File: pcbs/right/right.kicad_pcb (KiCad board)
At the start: 2 copper layers, 111.6 x 82.4 mm, 53 parts, among them J1 Conn_01x12_Socket

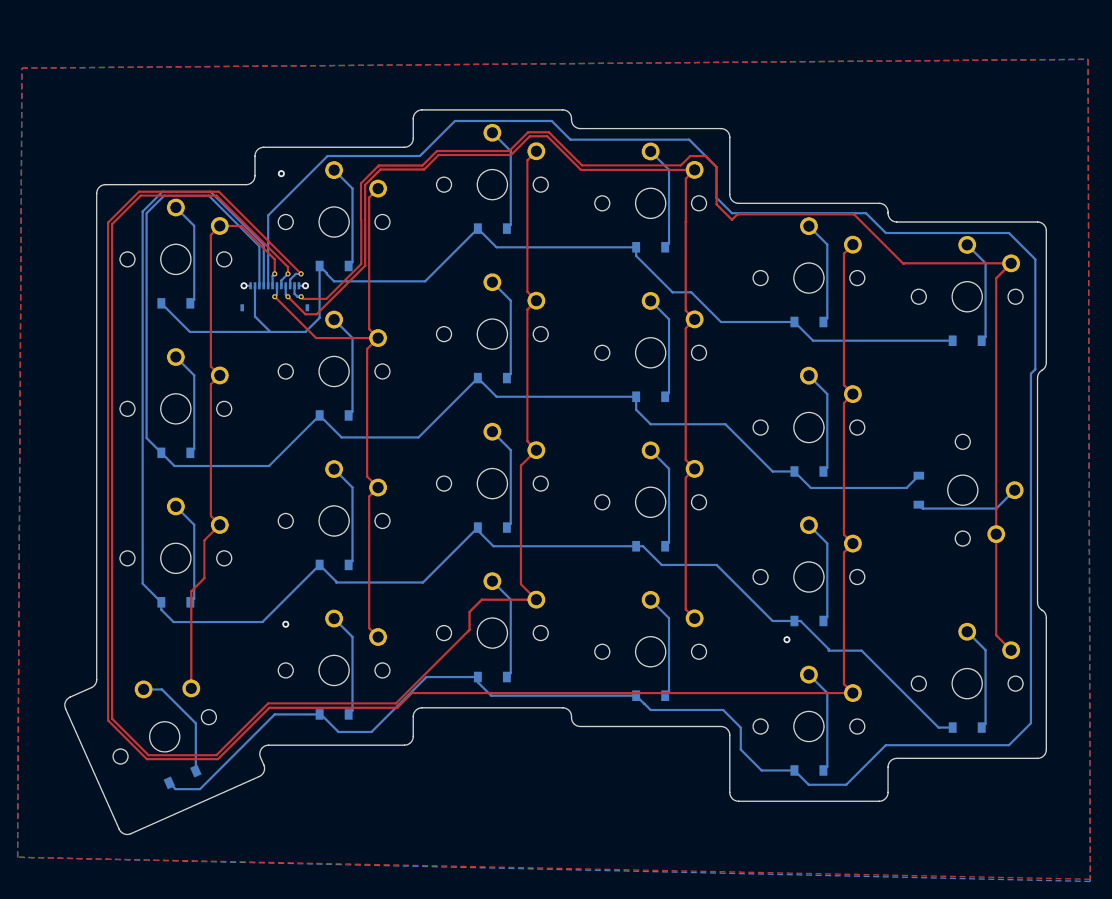
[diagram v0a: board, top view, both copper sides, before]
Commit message: fix offset etc
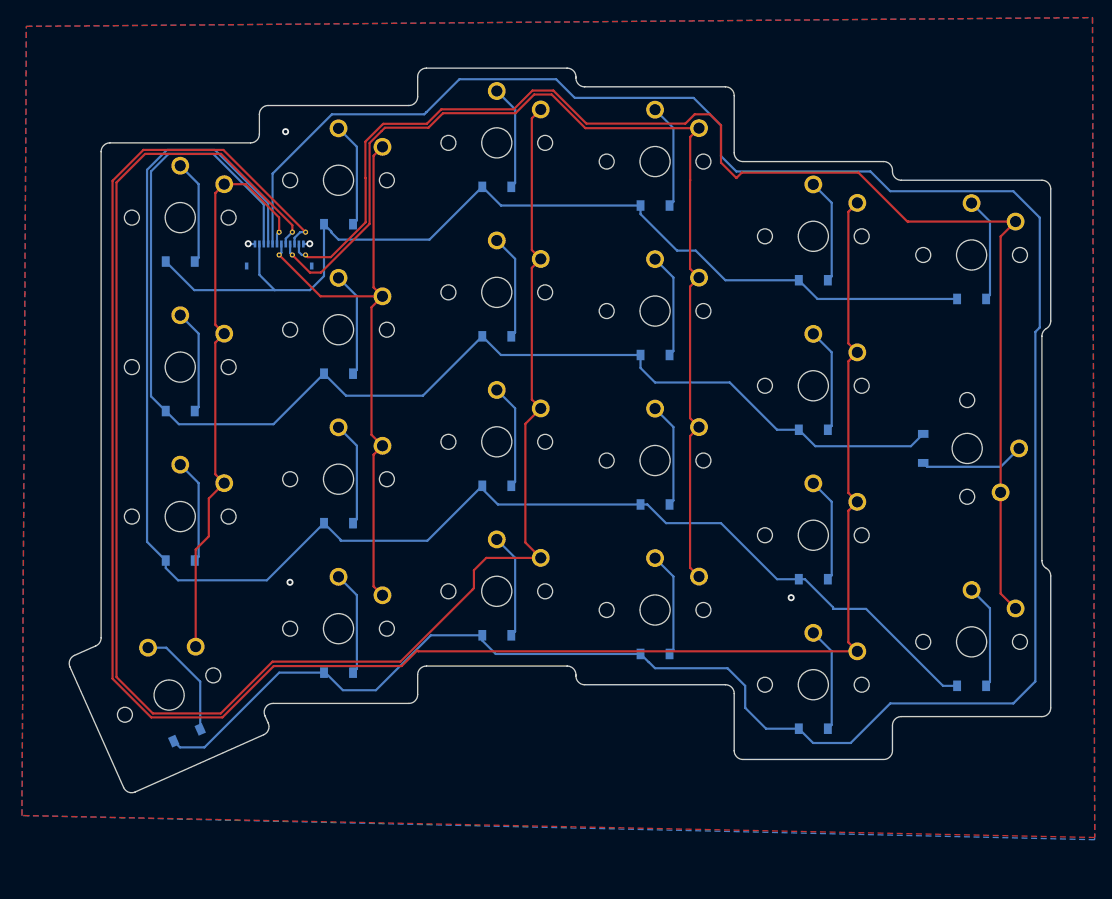
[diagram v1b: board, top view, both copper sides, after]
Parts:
- moved D1 4.78 mm to (316.0, 136.2)
- moved D10 4.78 mm to (280.0, 98.6)
- moved D11 4.78 mm to (280.0, 81.6)
- moved D12 4.78 mm to (262.0, 130.5)
- moved D13 4.78 mm to (262.0, 113.5)
- moved D14 4.78 mm to (262.0, 96.5)
- moved D15 4.78 mm to (262.0, 79.5)
- moved D16 4.78 mm to (244.0, 134.8)
- moved D17 4.78 mm to (244.0, 117.8)
- moved D18 4.78 mm to (244.0, 100.8)
- moved D19 4.78 mm to (244.0, 83.8)
- moved D2 4.78 mm to (310.5, 109.2)
- moved D20 4.78 mm to (226.8, 141.9)
- moved D21 4.78 mm to (226.0, 122.0)
- moved D22 4.78 mm to (226.0, 105.0)
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
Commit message: old changes
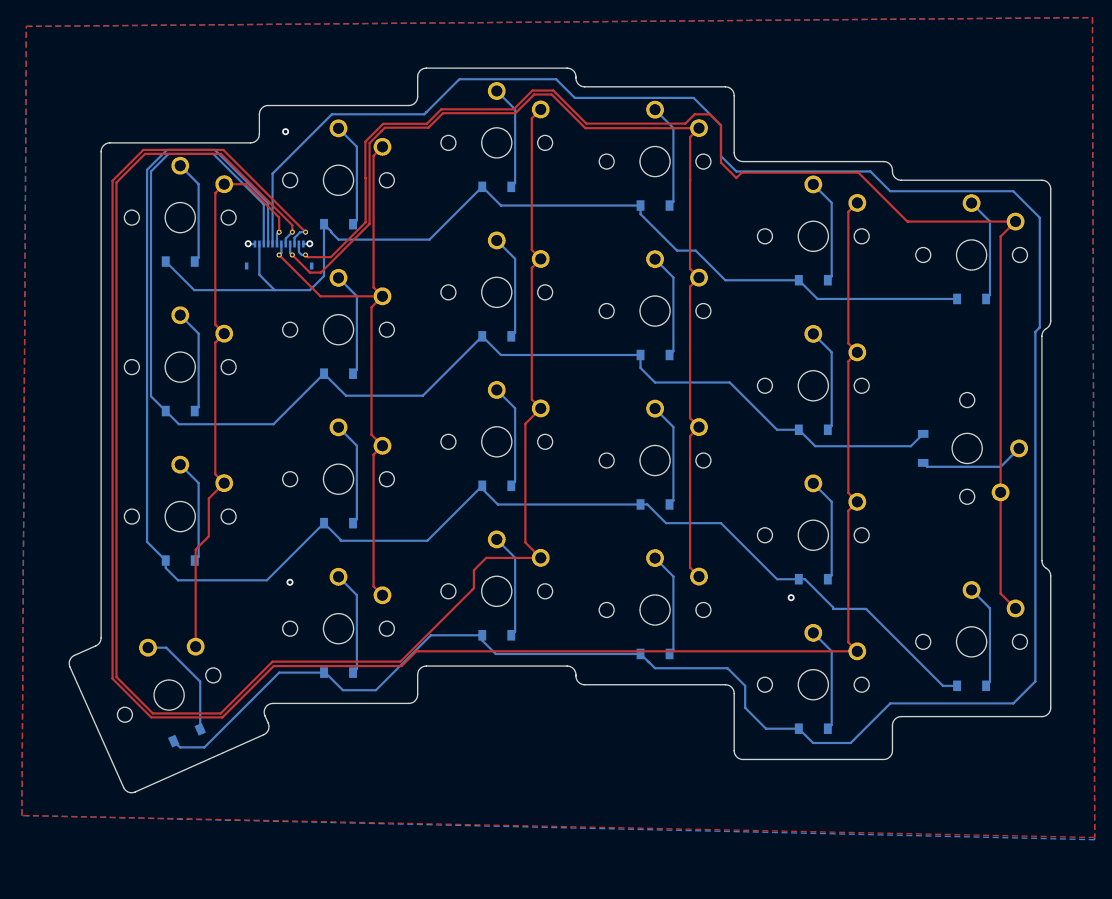
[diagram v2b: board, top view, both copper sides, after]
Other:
- net class Default added: clearance 0.2, trace_width 0.25, via_dia 0.8, via_drill 0.4
